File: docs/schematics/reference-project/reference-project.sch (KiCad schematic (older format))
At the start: 23 parts, among them J1 UART, Q1 MMBT3904, SW1 INPUT_0, SW2 INPUT_1, SW3 INPUT_2, SW4 INPUT_3, SW5 INPUT_4, SW6 INPUT_5, SW7 RESET, U1 74HC165D, U2 ATTINY85-20PU

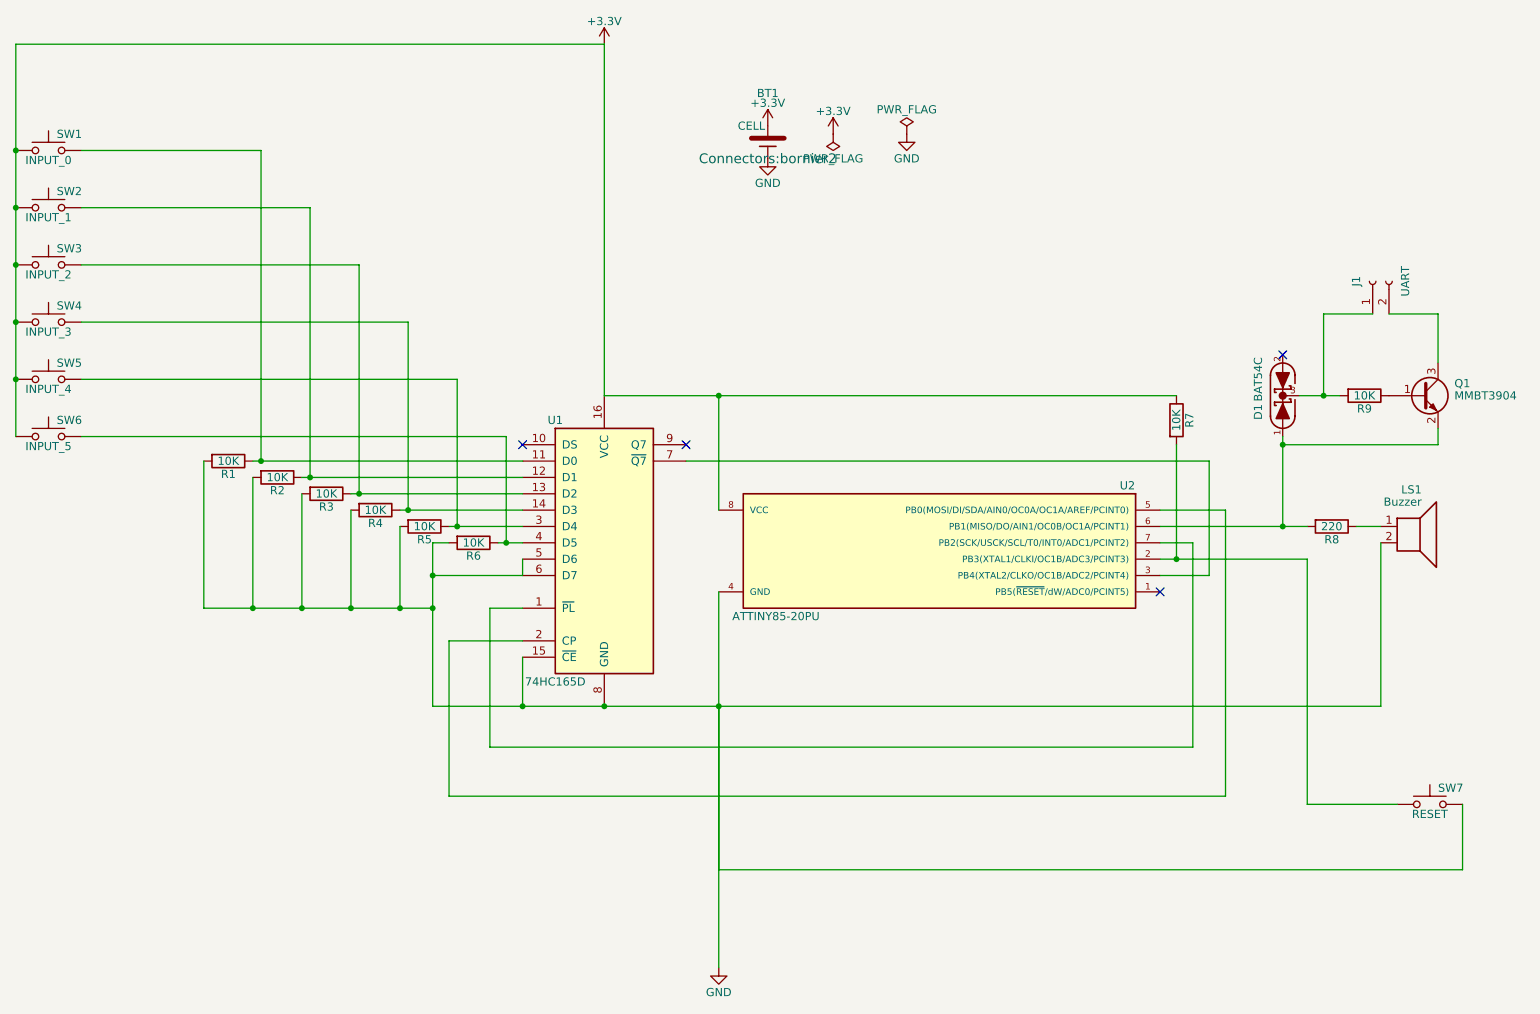
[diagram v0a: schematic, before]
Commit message: Updated to v3.
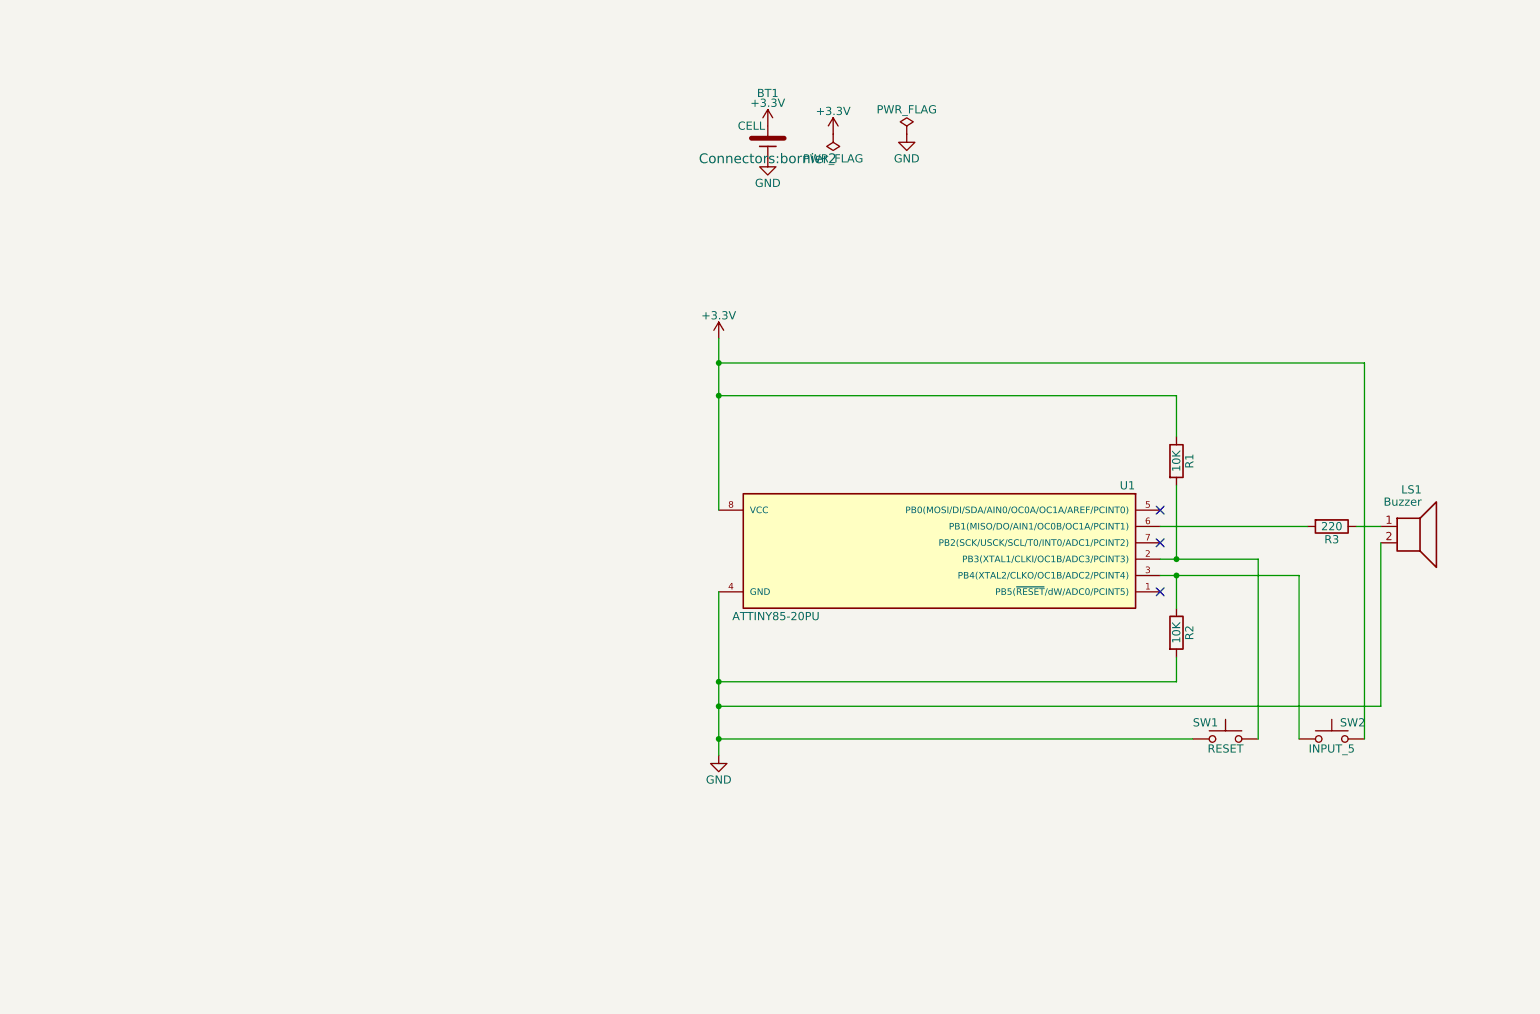
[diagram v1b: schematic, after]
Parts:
- removed D1: BAT54C, smd-semi:SOT-23, symbol BAT54C
- removed J1: UART, footprints:Header_2_Pin, symbol Conn_01x02_Female
- removed Q1: MMBT3904, TO_SOT_Packages_SMD:SOT-23, symbol MMBT3904
- removed R1, R2, R3, R4, R5, R9: 10K, Resistors_SMD:R_0805_HandSoldering, symbol R
- removed SW1: INPUT_0, Buttons_Switches_SMD:SW_SPST_TL3342, symbol SW_Push
- removed SW2: INPUT_1, Buttons_Switches_SMD:SW_SPST_TL3342, symbol SW_Push
- removed SW3: INPUT_2, Buttons_Switches_SMD:SW_SPST_TL3342, symbol SW_Push
- removed SW4: INPUT_3, Buttons_Switches_SMD:SW_SPST_TL3342, symbol SW_Push
- removed SW5: INPUT_4, Buttons_Switches_SMD:SW_SPST_TL3342, symbol SW_Push
- removed U1: 74HC165D, footprints:SOIC_16_0.154IN, symbol 74LS165
- renumbered R7 to R1, R6 to R2, R8 to R3, SW7 to SW1, SW6 to SW2, U2 to U1
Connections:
- net +3V3: now also SW2.2; no longer SW2.1
- net GND: now also SW1.1; no longer SW1.2
- net at R1.2, U1.2 (PB3(XTAL1/CLKI/OC1B/ADC3/PCINT3)): now also SW1.2; no longer SW1.1
- net at R2.1: now also SW2.1, U1.3 (PB4(XTAL2/CLKO/OC1B/ADC2/PCINT4)); no longer SW2.2
- no-connect marks 4 -> 3
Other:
- moved on the sheet: R1, R2, SW1, SW2
